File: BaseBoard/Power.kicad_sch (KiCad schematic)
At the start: 12 parts, among them J10 Conn_01x02_Female, J11 Conn_01x02_Female, J12 Conn_01x02_Female, J9 Barrel_Jack_Switch, K1 SRD-12V, U5 MINI560, U6 AMS1117-3.3

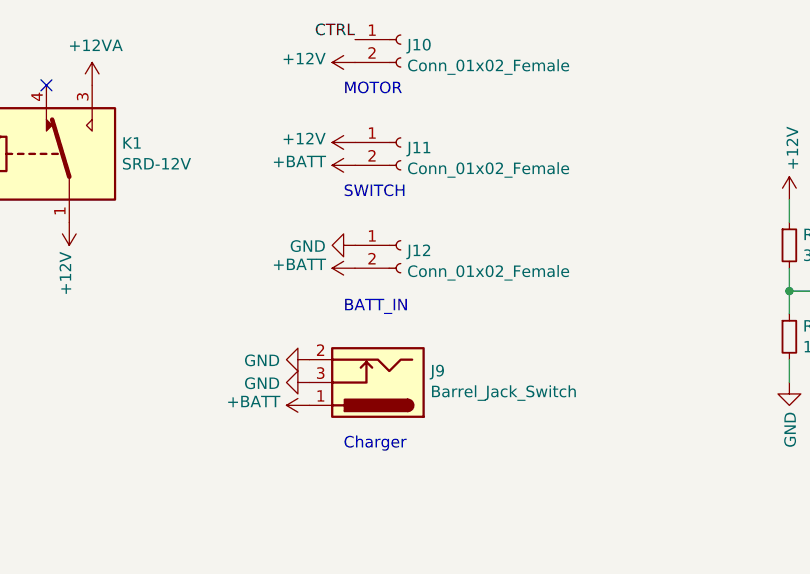
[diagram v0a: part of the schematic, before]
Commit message: 临时提交
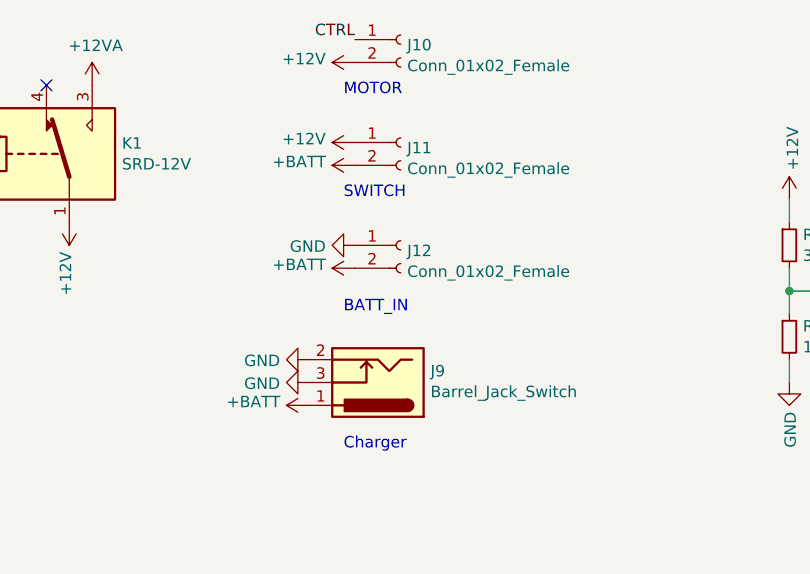
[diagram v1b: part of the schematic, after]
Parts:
- J10: footprint Connector_JST:JST_EH_S2B-EH_1x02_P2.50mm_Horizontal -> Connector_JST:JST_PH_S2B-PH-K_1x02_P2.00mm_Horizontal
- J11: footprint Connector_Molex:Molex_Mini-Fit_Jr_5569-02A2_2x01_P4.20mm_Horizontal -> Connector_Molex:Molex_KK-396_A-41792-0002_1x02_P3.96mm_Horizontal

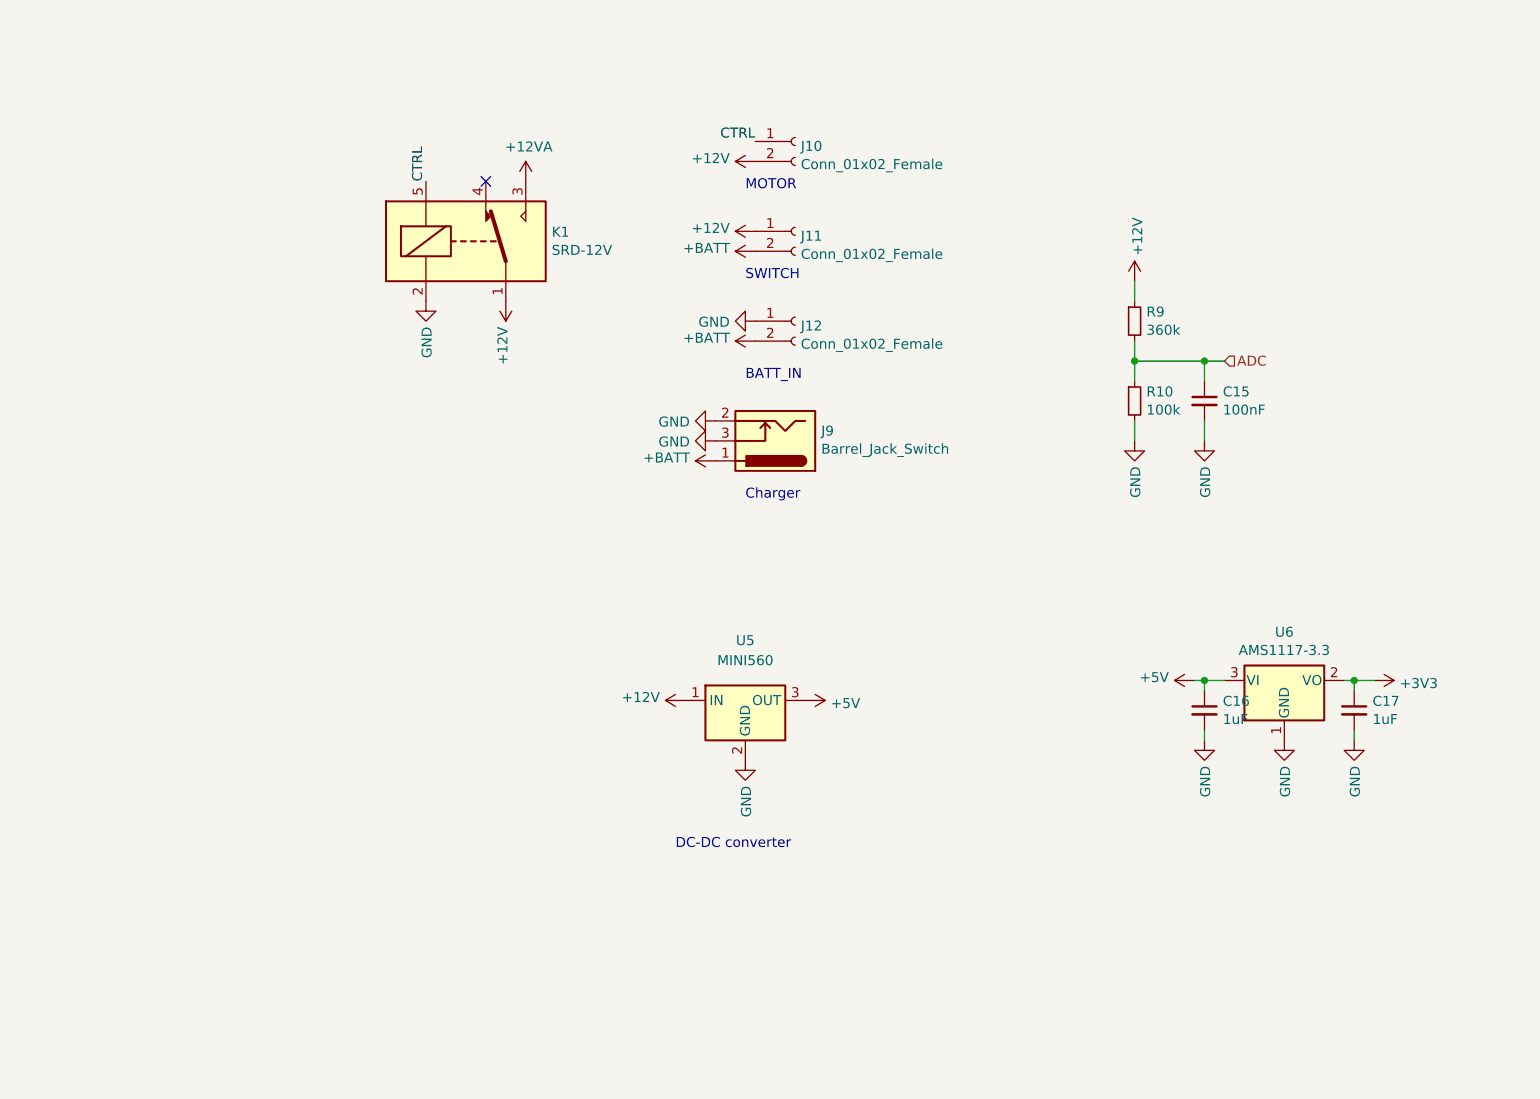
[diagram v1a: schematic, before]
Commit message: 更新V3线路板
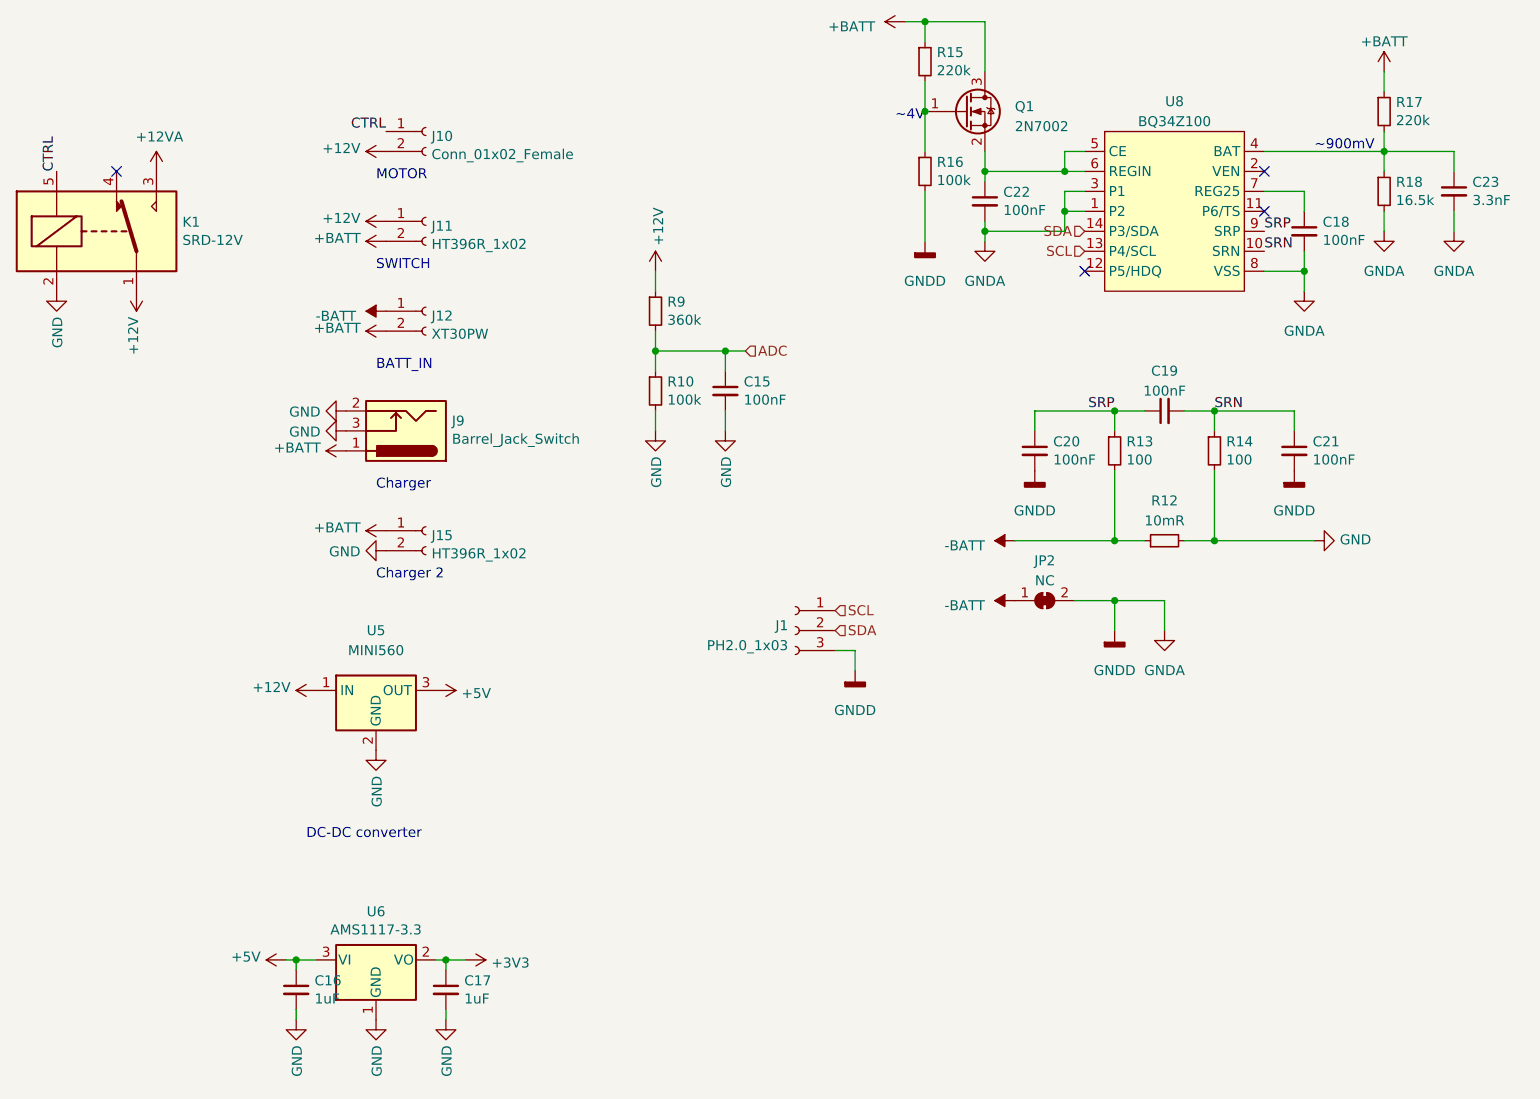
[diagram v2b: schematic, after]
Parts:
- added C18, C19, C20, C21, C22: 100nF, Capacitor_SMD:C_0805_2012Metric, symbol Device:C_Small
- added C23: 3.3nF, Capacitor_SMD:C_0805_2012Metric, symbol Device:C_Small
- added J1: PH2.0_1x03, Connector_JST:JST_PH_S3B-PH-K_1x03_P2.00mm_Horizontal, symbol Connector:Conn_01x03_Socket
- added J15: HT396R_1x02, Connector_Molex:Molex_KK-396_A-41792-0002_1x02_P3.96mm_Horizontal, symbol Connector:Conn_01x02_Female
- added JP2: NC, Jumper:SolderJumper-2_P1.3mm_Bridged2Bar_Pad1.0x1.5mm, symbol Jumper:SolderJumper_2_Bridged
- added Q1: 2N7002, Package_TO_SOT_SMD:SOT-23, symbol Transistor_FET:2N7002
- added R12: 10mR, Resistor_SMD:R_1210_3225Metric, symbol Device:R_Small
- added R13, R14: 100, Resistor_SMD:R_0805_2012Metric, symbol Device:R_Small
- added R15, R17: 220k, Resistor_SMD:R_0805_2012Metric, symbol Device:R_Small
- added R16: 100k, Resistor_SMD:R_0805_2012Metric, symbol Device:R_Small
- added R18: 16.5k, Resistor_SMD:R_0805_2012Metric, symbol Device:R_Small
- added U8: BQ34Z100, Package_SO:TSSOP-14_4.4x5mm_P0.65mm, symbol Smallbot:BQ34Z100
- J11: value Conn_01x02_Female -> HT396R_1x02
- J12: value Conn_01x02_Female -> XT30PW
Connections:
- net +BATT: now also J15.1 (Pin_1), Q1.3 (D), R15.1, R17.1
- net GND: now also J15.2 (Pin_2), R12.2, R14.2; no longer J12.1 (Pin_1)
- new net: Q1.1 (G), R15.2, R16.1
- new net: C22.1, Q1.2 (S), U8.5 (CE), U8.6 (REGIN)
- new net: C23.1, R17.2, R18.1, U8.4 (BAT)
- new net: C18.1, U8.7 (REG25)
- new net -BATT: J12.1 (Pin_1), JP2.1 (A), R12.1, R13.2
- new net GNDA: C18.2, C20.2, C21.2, C22.2, C23.2, J1.3 (Pin_3), JP2.2 (B), R16.2, R18.2, U8.1 (P2), U8.3 (P1), U8.8 (VSS)
- new net SCL: J1.1 (Pin_1), U8.13 (P4/SCL)
- new net SDA: J1.2 (Pin_2), U8.14 (P3/SDA)
- new net SRN: C19.2, C21.1, R14.1, U8.10 (SRN)
- new net SRP: C19.1, C20.1, R13.1, U8.9 (SRP)
- no-connect marks 1 -> 4
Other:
- note added: "Charger 2"
- note added: "~4V"
- note added: "~900mV"
- moved on the sheet: C15, C16, C17, J10, J11, J12, J9, K1, R10, R9, U5, U6
